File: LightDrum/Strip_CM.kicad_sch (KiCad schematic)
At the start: 10 parts, among them U42 INA4181 A2, U43 INA4181 A2

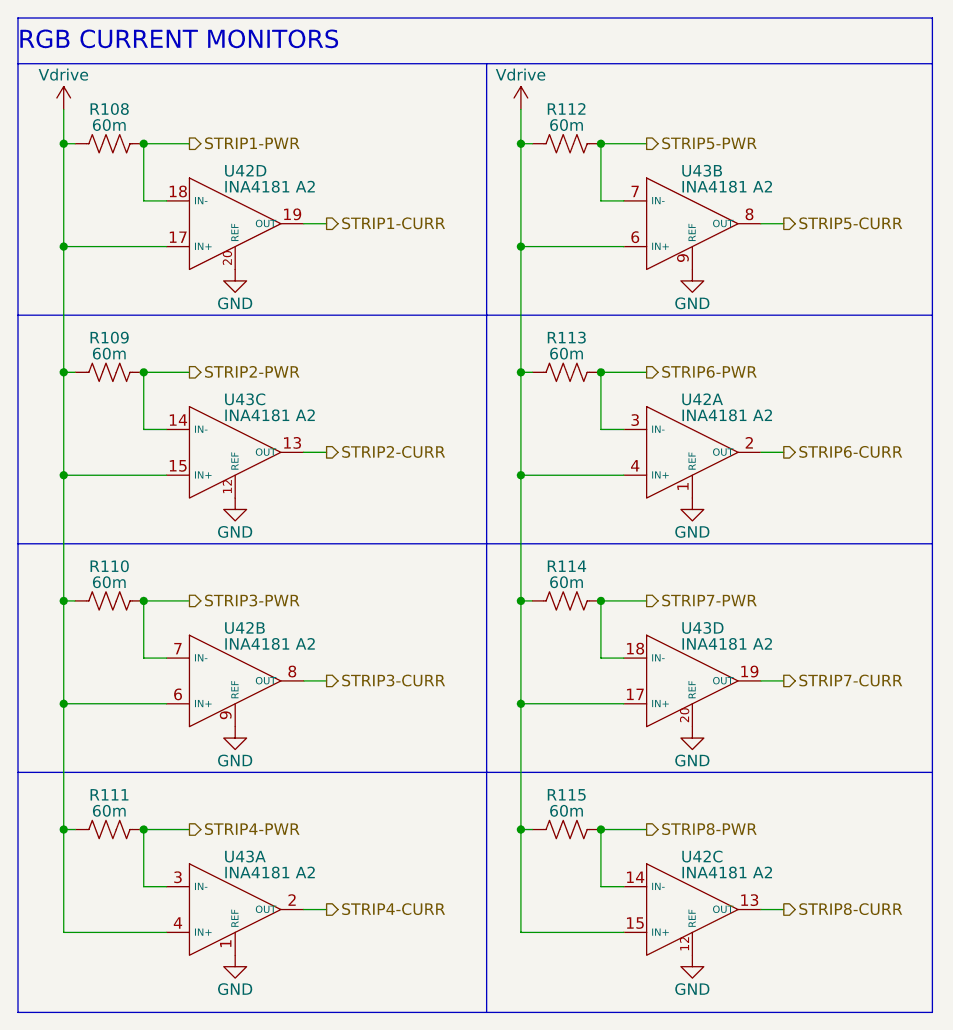
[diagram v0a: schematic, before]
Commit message: General component placement
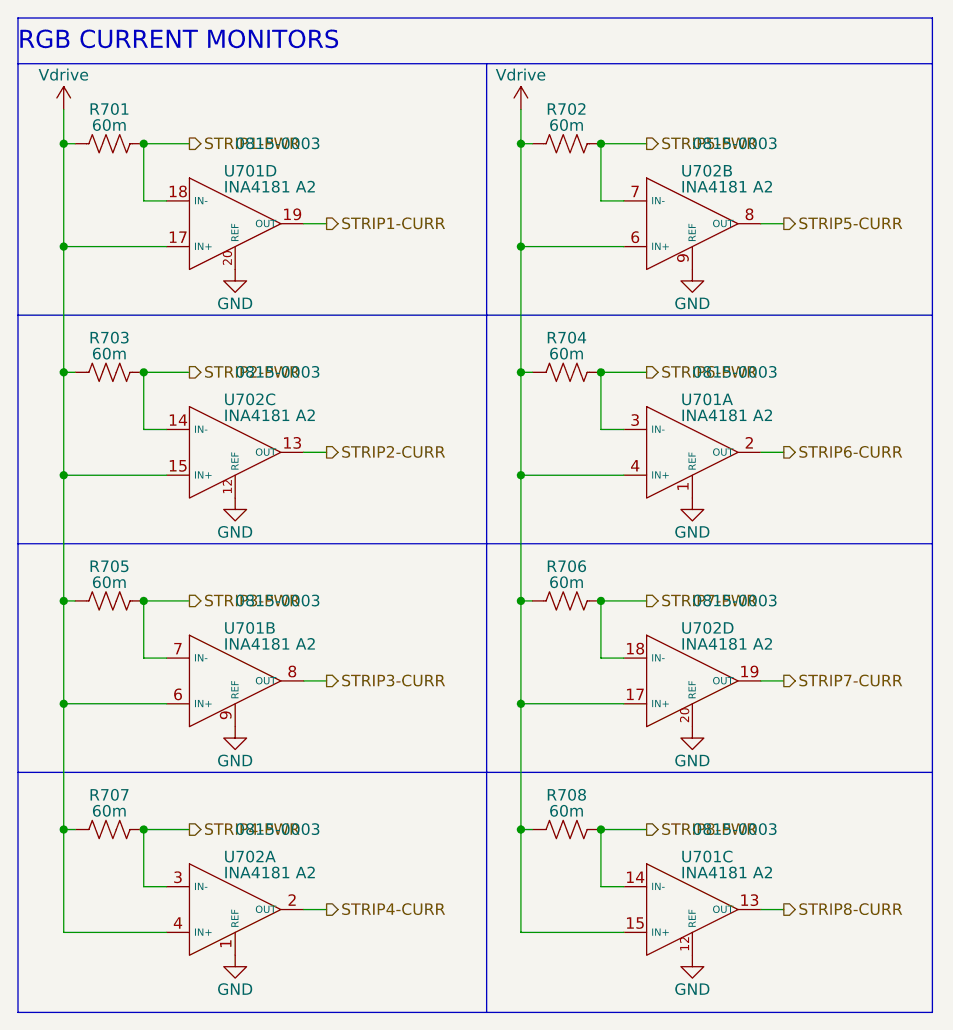
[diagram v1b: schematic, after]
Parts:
- U701: renamed from U42; PartNumber (none) -> 0815-0003
- U702: renamed from U43; PartNumber (none) -> 0815-0003
- renumbered R108 to R701, R112 to R702, R109 to R703, R113 to R704, R110 to R705, R114 to R706, R111 to R707, R115 to R708
